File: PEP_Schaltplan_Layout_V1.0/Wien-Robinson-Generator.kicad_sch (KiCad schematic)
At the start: 14 parts, among them Q5 BF256, U13 LT1819

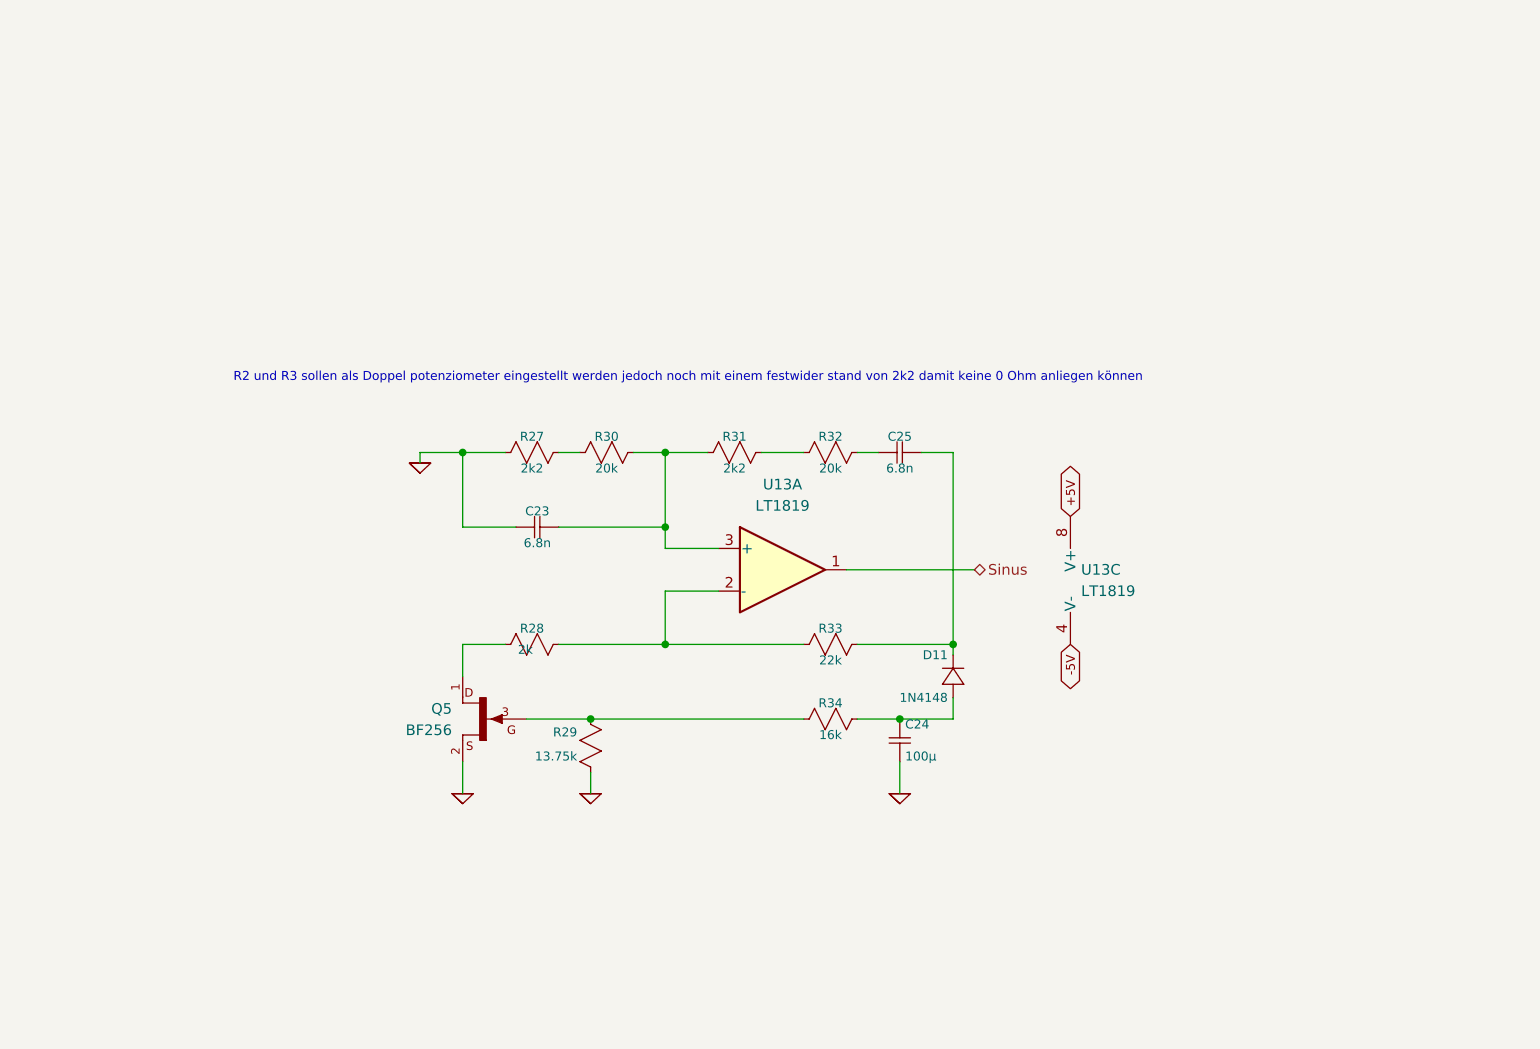
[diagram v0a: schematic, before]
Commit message: Bauoptionen1
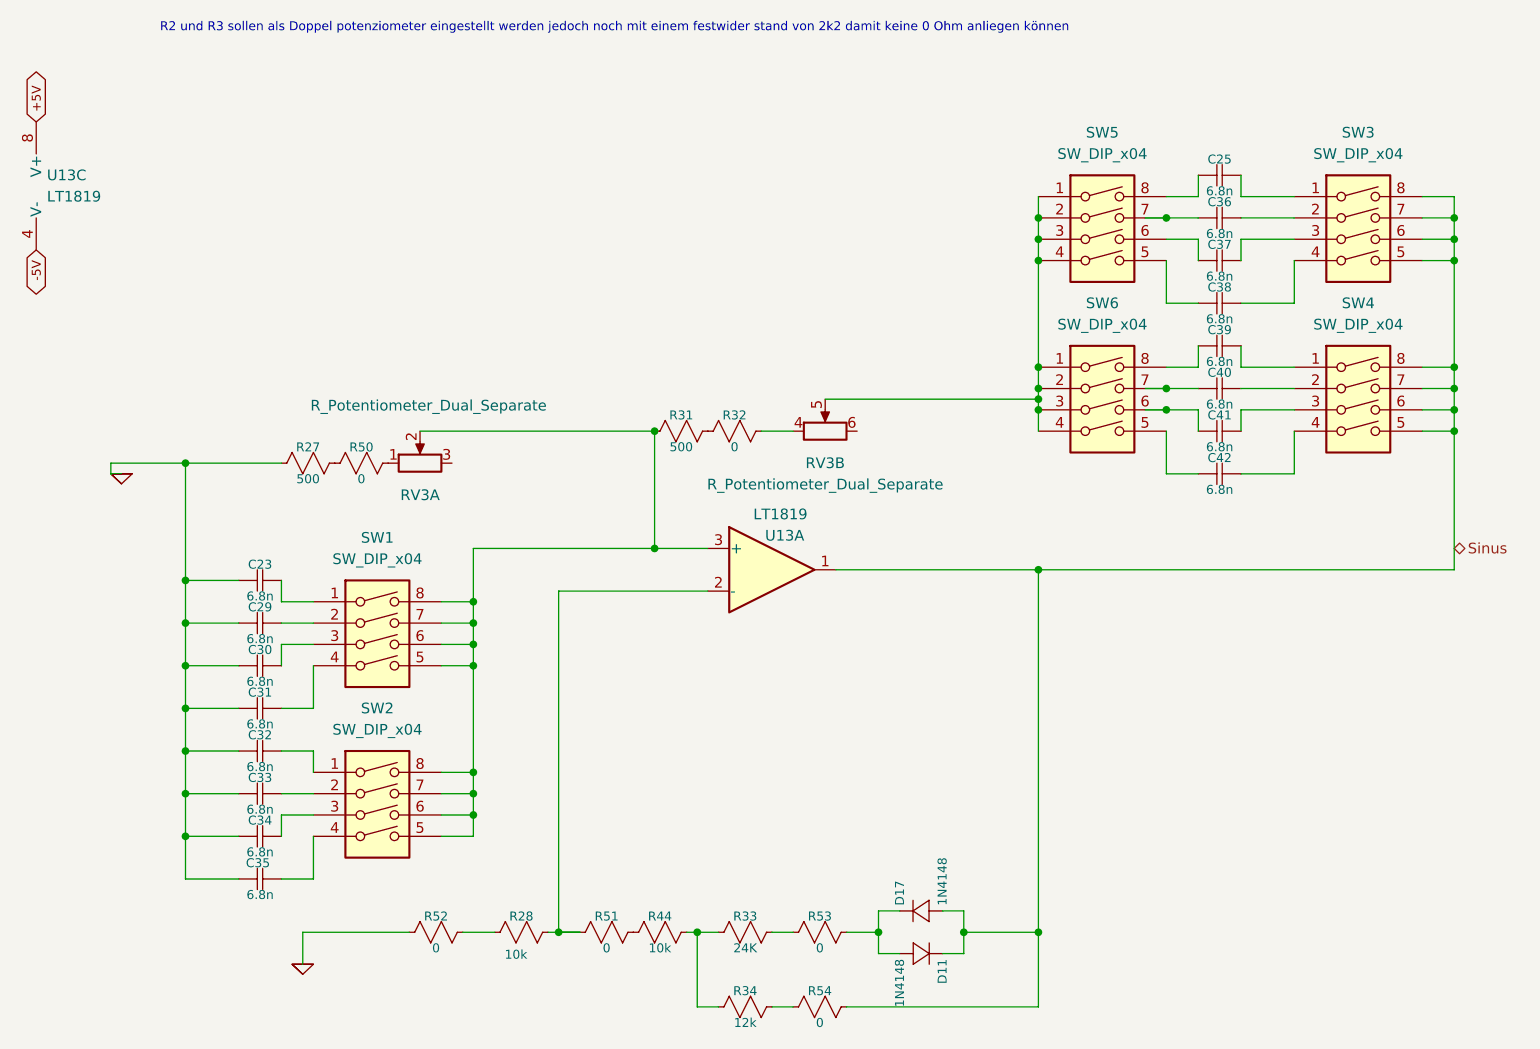
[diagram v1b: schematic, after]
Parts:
- removed C24: 100µ, Capacitor_THT:CP_Radial_D13.0mm_P5.00mm, symbol ltspice:cap
- removed Q5: BF256, Package_TO_SOT_THT:TO-92L_Inline, symbol BF256:BF256
- removed R29: 13.75k, Resistor_SMD:R_1206_3216Metric, symbol ltspice:res
- removed R30: 20k, Resistor_SMD:R_1206_3216Metric, symbol ltspice:res
- added C29, C30, C31, C32, C33, C34, C35, C36, C37, C38, C39, C40, C41, C42: 6.8n, Capacitor_SMD:C_1206_3216Metric, symbol ltspice:cap
- added D17: 1N4148, Diode_THT:D_DO-41_SOD81_P10.16mm_Horizontal, symbol ltspice:diode
- added R44: 10k, Resistor_SMD:R_1206_3216Metric, symbol ltspice:res
- added R50, R51, R52, R53, R54: 0, Resistor_SMD:R_1206_3216Metric, symbol ltspice:res
- added RV3: R_Potentiometer_Dual_Separate, Potentiometer_THT:Potentiometer_Piher_T-16H_Double_Horizontal, symbol Device:R_Potentiometer_Dual_Separate
- added SW1, SW2, SW3, SW4, SW5, SW6: SW_DIP_x04, Button_Switch_THT:SW_DIP_SPSTx04_Slide_6.7x11.72mm_W7.62mm_P2.54mm_LowProfile, symbol Switch:SW_DIP_x04
- R27, R31: value 2k2 -> 500
- R28: value 2k -> 10k
- R32: value 20k -> 0
- R33: value 22k -> 24K
- R34: value 16k -> 12k
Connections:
- net 0: now also C29.2, C30.2, C31.2, C32.2, C33.2, C34.2, C35.2, R52.2
- net Sinus: now also D11.2 (-), D17.1 (+), R54.1, SW3.5, SW3.6, SW3.7, SW3.8, SW4.5, SW4.6, SW4.7, SW4.8
- net at R31.2, U13.3 (+): now also RV3.2, SW1.5, SW1.6, SW1.7, SW1.8, SW2.5, SW2.6, SW2.7, SW2.8; no longer C23.1
- net at R34.2: now also R33.2, R44.1
- net at R27.1: now also R50.2
- net at R28.1, U13.2 (-): now also R51.2; no longer R33.2
- net at R28.2: now also R52.1
- net at C25.2: now also SW5.8; no longer R32.1
- net at D11.1 (+): now also D17.2 (-), R53.1; no longer R34.1
- new net: C39.1, SW4.1
- new net: C40.1, SW4.2
- new net: C41.1, SW4.3
- new net: C42.1, SW4.4
- new net: C23.1, SW1.1
- new net: C30.1, SW1.3
- new net: R33.1, R53.2
- new net: C32.1, SW2.1
- new net: C35.1, SW2.4
- new net: C36.1, SW3.2
- new net: C36.2, SW5.7
- new net: C25.1, SW3.1
- new net: R32.1, RV3.4
- new net: RV3.5, SW5.1, SW5.2, SW5.3, SW5.4, SW6.1, SW6.2, SW6.3, SW6.4
- new net: R50.1, RV3.1
- new net: R44.2, R51.1
- new net: C31.1, SW1.4
- new net: C38.2, SW5.5
- new net: C37.2, SW5.6
- new net: C39.2, SW6.8
- new net: C42.2, SW6.5
- new net: C33.1, SW2.2
- new net: C40.2, SW6.7
- new net: C37.1, SW3.3
- new net: C29.1, SW1.2
- new net: R34.1, R54.2
- new net: C38.1, SW3.4
- new net: C34.1, SW2.3
- new net: C41.2, SW6.6
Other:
- moved on the sheet: C23, D11, R27, R28, R31, R33, R34, U13A, U13C
